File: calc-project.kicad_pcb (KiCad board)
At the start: 2 copper layers, 80 x 100 mm, 68 parts, among them J1 PinSocket_1x20_Right, J2 PinSocket_1x20_Left, J3 Conn_01x14, SW1 SW_Push_45deg, SW10 SW_Push_45deg, SW11 SW_Push_45deg, SW12 SW_Push_45deg, SW13 SW_Push_45deg, SW14 SW_Push_45deg, SW15 SW_Push_45deg, SW16 SW_Push_45deg, SW17 SW_Push_45deg, SW18 SW_Push_45deg, SW19 SW_Push_45deg, SW2 SW_Push_45deg, SW20 SW_Push_45deg, SW21 SW_Push_45deg, SW22 SW_Push_45deg, SW23 SW_Push_45deg, SW24 SW_Push_45deg, SW25 SW_Push_45deg, SW26 SW_Push_45deg, SW27 SW_Push_45deg, SW28 SW_Push_45deg, SW29 SW_Push_45deg, SW3 SW_Push_45deg, SW30 SW_Push_45deg, SW31 SW_Push_45deg, SW32 SW_Push_45deg, SW33 SW_Push_45deg, SW34 SW_Push_45deg, SW35 SW_Push_45deg, SW36 SW_Push_45deg, SW4 SW_Push_45deg, SW5 SW_Push_45deg, SW6 SW_Push_45deg, SW7 SW_Push_45deg, SW8 SW_Push_45deg, SW9 SW_Push_45deg

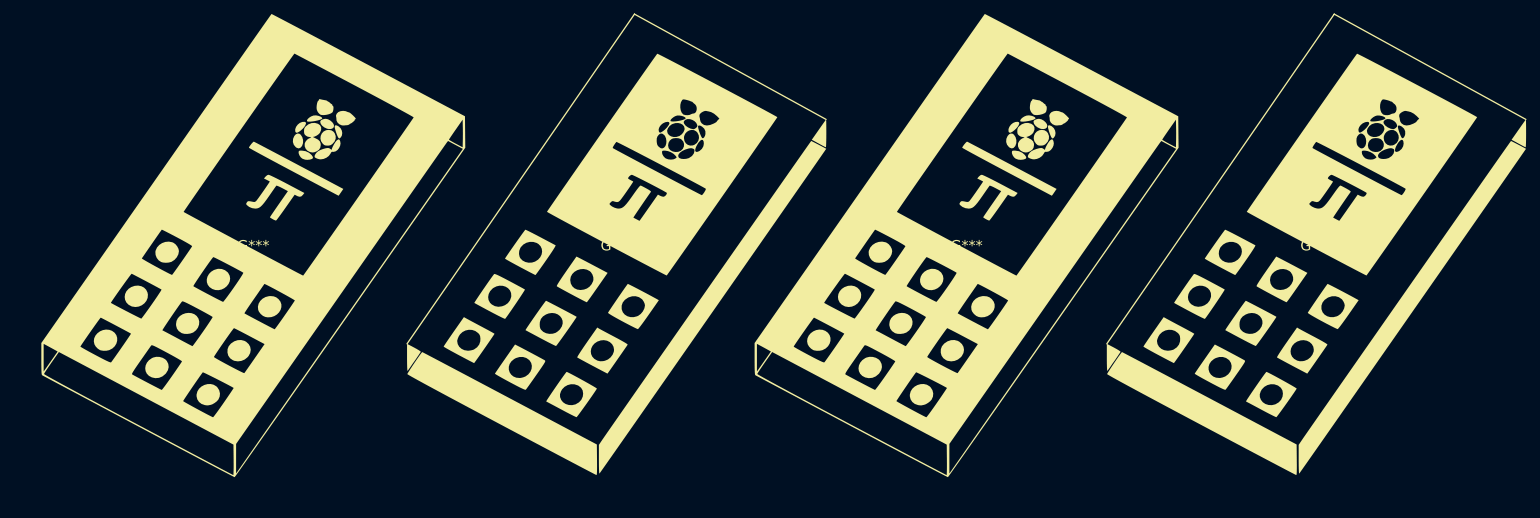
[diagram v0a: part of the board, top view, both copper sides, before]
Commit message: idek what just happened
but im trusting its fine
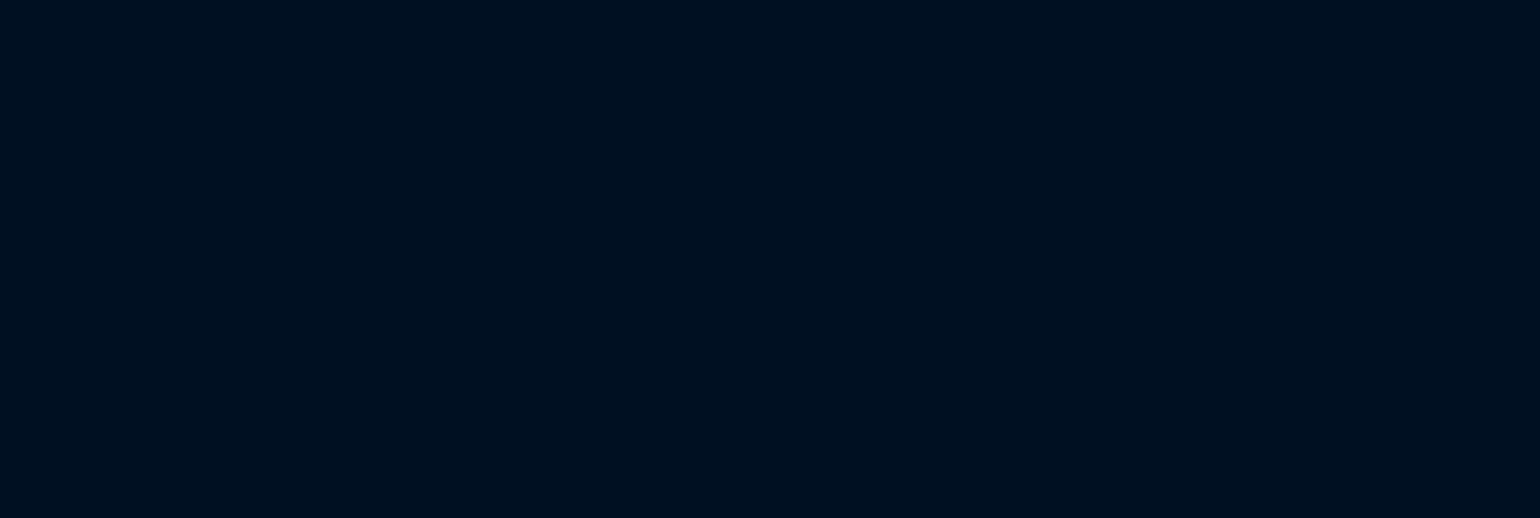
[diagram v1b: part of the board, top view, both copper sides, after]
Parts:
- removed the G*** at (228.6, 101.6)
- removed the G*** at (279.4, 101.6)
- removed the G*** at (330.2, 101.6)
- removed the G*** at (175.8, 101.6)
